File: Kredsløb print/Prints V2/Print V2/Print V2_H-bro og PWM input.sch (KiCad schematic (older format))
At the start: 19 parts, among them J1 Conn_01x01_Male, J19 Conn_01x01_Male, J2 Conn_01x01_Male, J20 Conn_01x01_Male, J28 Conn_01x01_Male, J3 Conn_01x01_Male, J30 Conn_01x01_Male, J4 Conn_01x01_Male, J5 Conn_01x01_Male, Q17 BC547, Q20 BC547, Q21 TIP127, Q22 TIP120, Q24 TIP120, Q27 TIP127, Q28 TIP120

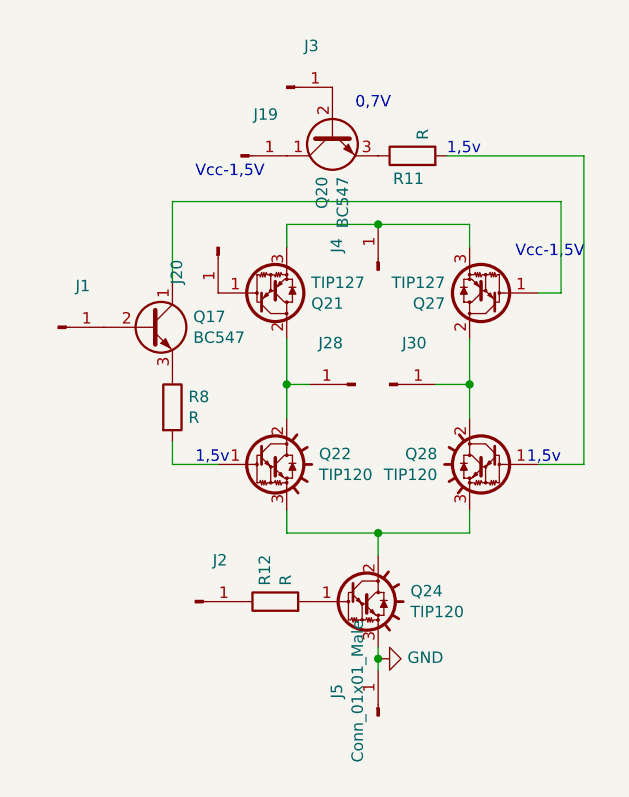
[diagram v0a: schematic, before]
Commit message: Stuff
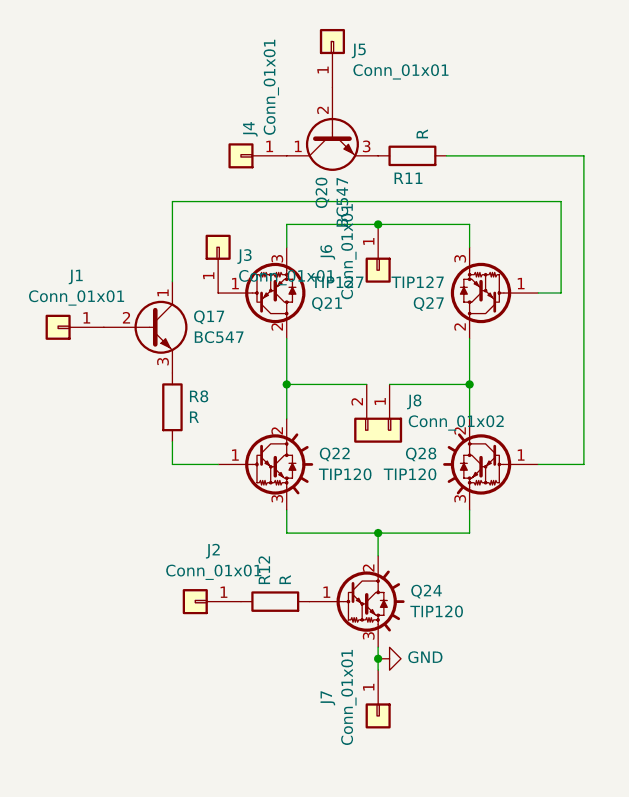
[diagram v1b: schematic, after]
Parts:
- removed J1, J19, J2, J20, J28, J3, J30, J4, J5: Conn_01x01_Male, Connector_PinHeader_2.54mm:PinHeader_1x01_P2.54mm_Vertical, symbol Connector:Conn_01x01_Male
- added J1, J2, J3, J4, J5, J6, J7: Conn_01x01, Custom footprints:Wire_hole, symbol Connector_Generic:Conn_01x01
- added J8: Conn_01x02, Connector_PinSocket_2.54mm:PinSocket_1x02_P2.54mm_Vertical, symbol Connector_Generic:Conn_01x02
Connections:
- net GND: now also J7.1 (Pin_1)
- net at Q21.3 (E), Q27.3 (E): now also J6.1 (Pin_1)
- net at Q17.2 (B): now also J1.1 (Pin_1)
- net at Q20.2 (B): now also J5.1 (Pin_1)
- net at R12.1: now also J2.1 (Pin_1)
- net at Q21.2 (C), Q22.2 (C): now also J8.2 (Pin_2)
- net at Q27.2 (C), Q28.2 (C): now also J8.1 (Pin_1)
- net at Q20.1 (C): now also J4.1 (Pin_1)
- net at Q21.1 (B): now also J3.1 (Pin_1)
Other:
- note removed: "0,7V"
- note removed: "1,5v"
- note removed: "Vcc-1,5V"
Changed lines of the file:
@@
 	1    0    0    -1
 $EndComp
-$Comp
-L Connector:Conn_01x01_Male J30
-U 1 1 5CB310DE
-P 5650 3350
-F 0 "J30" H 5758 3531 50  0000 C CNN
-F 1 "Conn_01x01_Male" H 5758 3440 50  0001 C CNN
-F 2 "Connector_PinHeader_2.54mm:PinHeader_1x01_P2.54mm_Vertical" H 5650 3350 50  0001 C CNN
-F 3 "~" H 5650 3350 50  0001 C CNN
-	1    5650 3350
-	1    0    0    -1
-$EndComp
 Connection ~ 6000 3350
 Wire Wire Line
 	6000 3350 6000 3500
-$Comp
-L Connector:Conn_01x01_Male J28
-U 1 1 5CB310E6
-P 5500 3350
-F 0 "J28" H 5608 3531 50  0000 C CNN
-F 1 "Conn_01x01_Male" H 5608 3440 50  0001 C CNN
-F 2 "Connector_PinHeader_2.54mm:PinHeader_1x01_P2.54mm_Vertical" H 5500 3350 50  0001 C CNN
-F 3 "~" H 5500 3350 50  0001 C CNN
-	1    5500 3350
-	-1   0    0    -1
-$EndComp
-Wire Wire Line
-	5300 3350 5200 3350
 Connection ~ 5200 3350
 Wire Wire Line
@@
 	4700 3700 4700 3600
 $Comp
-L Connector:Conn_01x01_Male J20
-U 1 1 5CB3112E
-P 4900 2750
-F 0 "J20" H 5008 2931 50  0000 C CNN
-F 1 "Conn_01x01_Male" H 5008 2840 50  0001 C CNN
-F 2 "Connector_PinHeader_2.54mm:PinHeader_1x01_P2.54mm_Vertical" H 4900 2750 50  0001 C CNN
-F 3 "~" H 4900 2750 50  0001 C CNN
-	1    4900 2750
-	0    -1   1    0
-$EndComp
-$Comp
-L Connector:Conn_01x01_Male J19
-U 1 1 5CB31134
-P 5000 2350
-F 0 "J19" H 5108 2531 50  0000 C CNN
-F 1 "Conn_01x01_Male" H 5108 2440 50  0001 C CNN
-F 2 "Connector_PinHeader_2.54mm:PinHeader_1x01_P2.54mm_Vertical" H 5000 2350 50  0001 C CNN
-F 3 "~" H 5000 2350 50  0001 C CNN
-	1    5000 2350
-	1    0    0    -1
-$EndComp
-Wire Wire Line
-	5850 3350 6000 3350
-$Comp
 L Device:R R12
 U 1 1 5CB3113B
@@
 	5600 4600 5600 4550
 Wire Wire Line
-	5200 2650 5600 2650
-Wire Wire Line
 	6400 2950 6300 2950
 $Comp
@@
 	-1   0    0    1
 $EndComp
-Connection ~ 5600 2650
-Wire Wire Line
-	5600 2650 6000 2650
-$Comp
-L Connector:Conn_01x01_Male J4
-U 1 1 5CAE1552
-P 5600 2850
-F 0 "J4" H 5708 3031 50  0000 C CNN
-F 1 "Conn_01x01_Male" H 5708 2940 50  0001 C CNN
-F 2 "Connector_PinHeader_2.54mm:PinHeader_1x01_P2.54mm_Vertical" H 5600 2850 50  0001 C CNN
-F 3 "~" H 5600 2850 50  0001 C CNN
-	1    5600 2850
-	0    -1   -1   0
-$EndComp
 Wire Wire Line
 	4700 2550 6400 2550
@@
 Wire Wire Line
 	5600 4100 5600 4000
-$Comp
-L Connector:Conn_01x01_Male J1
-U 1 1 5CAEBDCC
-P 4200 3100
-F 0 "J1" H 4308 3281 50  0000 C CNN
-F 1 "Conn_01x01_Male" H 4308 3190 50  0001 C CNN
-F 2 "Connector_PinHeader_2.54mm:PinHeader_1x01_P2.54mm_Vertical" H 4200 3100 50  0001 C CNN
-F 3 "~" H 4200 3100 50  0001 C CNN
-	1    4200 3100
-	1    0    0    -1
-$EndComp
-$Comp
-L Connector:Conn_01x01_Male J3
-U 1 1 5CAEC4E3
-P 5200 2050
-F 0 "J3" H 5308 2231 50  0000 C CNN
-F 1 "Conn_01x01_Male" H 5308 2140 50  0001 C CNN
-F 2 "Connector_PinHeader_2.54mm:PinHeader_1x01_P2.54mm_Vertical" H 5200 2050 50  0001 C CNN
-F 3 "~" H 5200 2050 50  0001 C CNN
-	1    5200 2050
-	1    0    0    -1
-$EndComp
-$Comp
-L Connector:Conn_01x01_Male J2
-U 1 1 5CAECC3B
-P 4800 4300
-F 0 "J2" H 4908 4481 50  0000 C CNN
-F 1 "Conn_01x01_Male" H 4908 4390 50  0001 C CNN
-F 2 "Connector_PinHeader_2.54mm:PinHeader_1x01_P2.54mm_Vertical" H 4800 4300 50  0001 C CNN
-F 3 "~" H 4800 4300 50  0001 C CNN
-	1    4800 4300
-	1    0    0    -1
-$EndComp
-$Comp
-L Connector:Conn_01x01_Male J5
-U 1 1 5CAED36D
-P 5600 4800
-F 0 "J5" H 5708 4981 50  0000 C CNN
-F 1 "Conn_01x01_Male" H 5708 4890 50  0000 C CNN
-F 2 "Connector_PinHeader_2.54mm:PinHeader_1x01_P2.54mm_Vertical" H 5600 4800 50  0001 C CNN
-F 3 "~" H 5600 4800 50  0001 C CNN
-	1    5600 4800
-	0    -1   -1   0
-$EndComp
 $Comp
 L power:GND #PWR0101
@@
 Wire Wire Line
 	5600 4550 5600 4500
-Text Notes 4800 2450 0    50   ~ 0
-Vcc-1,5V
-Text Notes 6250 3700 0    50   ~ 0
-1,5v
-Text Notes 5900 2350 0    50   ~ 0
-1,5v
-Text Notes 5500 2150 0    50   ~ 0
-0,7V
-Text Notes 6200 2800 0    50   ~ 0
-Vcc-1,5V
-Text Notes 4800 3700 0    50   ~ 0
-1,5v
+$Comp
+L Connector_Generic:Conn_01x02 J8
+U 1 1 5CC72A14
+P 5650 3550
+F 0 "J8" V 5522 3630 50  0000 L CNN
+F 1 "Conn_01x02" V 5613 3630 50  0000 L CNN
+F 2 "Connector_PinSocket_2.54mm:PinSocket_1x02_P2.54mm_Vertical" H 5650 3550 50  0001 C CNN
+F 3 "~" H 5650 3550 50  0001 C CNN
+	1    5650 3550
+	0    1    1    0
+$EndComp
+Wire Wire Line
+	5650 3350 6000 3350
+Wire Wire Line
+	5200 3350 5550 3350
+$Comp
+L Connector_Generic:Conn_01x01 J5
+U 1 1 5CC7573F
+P 5400 1850
+F 0 "J5" V 5364 1762 50  0000 R CNN
+F 1 "Conn_01x01" V 5273 1762 50  0000 R CNN
+F 2 "Custom footprints:Wire_hole" H 5400 1850 50  0001 C CNN
+F 3 "~" H 5400 1850 50  0001 C CNN
+	1    5400 1850
+	0    -1   -1   0
+$EndComp
+$Comp
+L Connector_Generic:Conn_01x01 J1
+U 1 1 5CC7650F
+P 4200 3100
+F 0 "J1" H 4118 2875 50  0000 C CNN
+F 1 "Conn_01x01" H 4118 2966 50  0000 C CNN
+F 2 "Custom footprints:Wire_hole" H 4200 3100 50  0001 C CNN
+F 3 "~" H 4200 3100 50  0001 C CNN
+	1    4200 3100
+	-1   0    0    1
+$EndComp
+$Comp
+L Connector_Generic:Conn_01x01 J6
+U 1 1 5CC784BA
+P 5600 2850
+F 0 "J6" H 5518 2625 50  0000 C CNN
+F 1 "Conn_01x01" H 5518 2716 50  0000 C CNN
+F 2 "Custom footprints:Wire_hole" H 5600 2850 50  0001 C CNN
+F 3 "~" H 5600 2850 50  0001 C CNN
+	1    5600 2850
+	0    1    1    0
+$EndComp
+$Comp
+L Connector_Generic:Conn_01x01 J2
+U 1 1 5CC789E3
+P 4800 4300
+F 0 "J2" H 4718 4075 50  0000 C CNN
+F 1 "Conn_01x01" H 4718 4166 50  0000 C CNN
+F 2 "Custom footprints:Wire_hole" H 4800 4300 50  0001 C CNN
+F 3 "~" H 4800 4300 50  0001 C CNN
+	1    4800 4300
+	-1   0    0    1
+$EndComp
+$Comp
+L Connector_Generic:Conn_01x01 J7
+U 1 1 5CC78D4E
+P 5600 4800
+F 0 "J7" H 5518 4575 50  0000 C CNN
+F 1 "Conn_01x01" H 5518 4666 50  0000 C CNN
+F 2 "Custom footprints:Wire_hole" H 5600 4800 50  0001 C CNN
+F 3 "~" H 5600 4800 50  0001 C CNN
+	1    5600 4800
+	0    1    1    0
+$EndComp
+Wire Wire Line
+	5200 2650 5600 2650
+Connection ~ 5600 2650
+Wire Wire Line
+	5600 2650 6000 2650
+$Comp
+L Connector_Generic:Conn_01x01 J4
+U 1 1 5CC7CE50
+P 5000 2350
+F 0 "J4" V 4964 2262 50  0000 R CNN
+F 1 "Conn_01x01" V 4873 2262 50  0000 R CNN
+F 2 "Custom footprints:Wire_hole" H 5000 2350 50  0001 C CNN
+F 3 "~" H 5000 2350 50  0001 C CNN
+	1    5000 2350
+	-1   0    0    1
+$EndComp
+$Comp
+L Connector_Generic:Conn_01x01 J3
+U 1 1 5CC7DC02
+P 4900 2750
+F 0 "J3" V 4864 2662 50  0000 R CNN
+F 1 "Conn_01x01" V 4773 2662 50  0000 R CNN
+F 2 "Custom footprints:Wire_hole" H 4900 2750 50  0001 C CNN
+F 3 "~" H 4900 2750 50  0001 C CNN
+	1    4900 2750
+	0    -1   -1   0
+$EndComp
 $EndSCHEMATC
